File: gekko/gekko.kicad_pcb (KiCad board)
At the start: 2 copper layers, 58 x 60.5 mm, 89 parts, among them J1 Conn_01x02_Male, J2 Conn_01x04_Female, J3 Conn_01x05, J4 Conn_01x03, J5 Conn_01x02_Male, J6 Conn_01x02, J7 Conn_01x04_Female, J8 Conn_01x02_Male, J9 Conn_01x02_Male, Q5 IRLML6344TRPBFTR, SW1 SW_Push_Dual_x2, SW2 SW_DPDT_x2, U1 DRV8835, U10 MA702GQ-P, U11 MA702GQ-P, U12 sw_pch, U2 STM32F413CH6, U3 LED_FOTR, U4 LP5907_DBV, U5 ICM20648, U6 LED_FOTR, U7 LED_FOTR, U8 LED_FOTR, U9 RP124N334E-TR-FE, Y1 Crystal_GND23

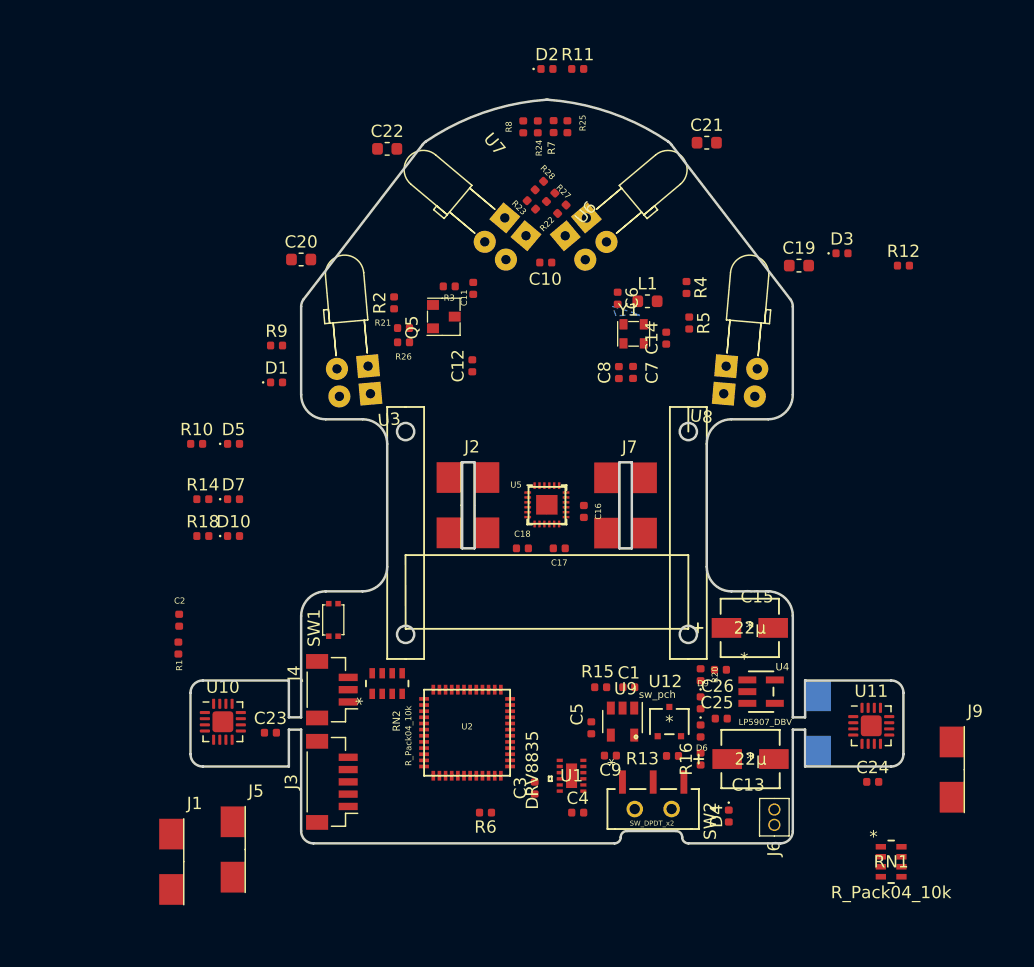
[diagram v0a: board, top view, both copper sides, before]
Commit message: betaGND
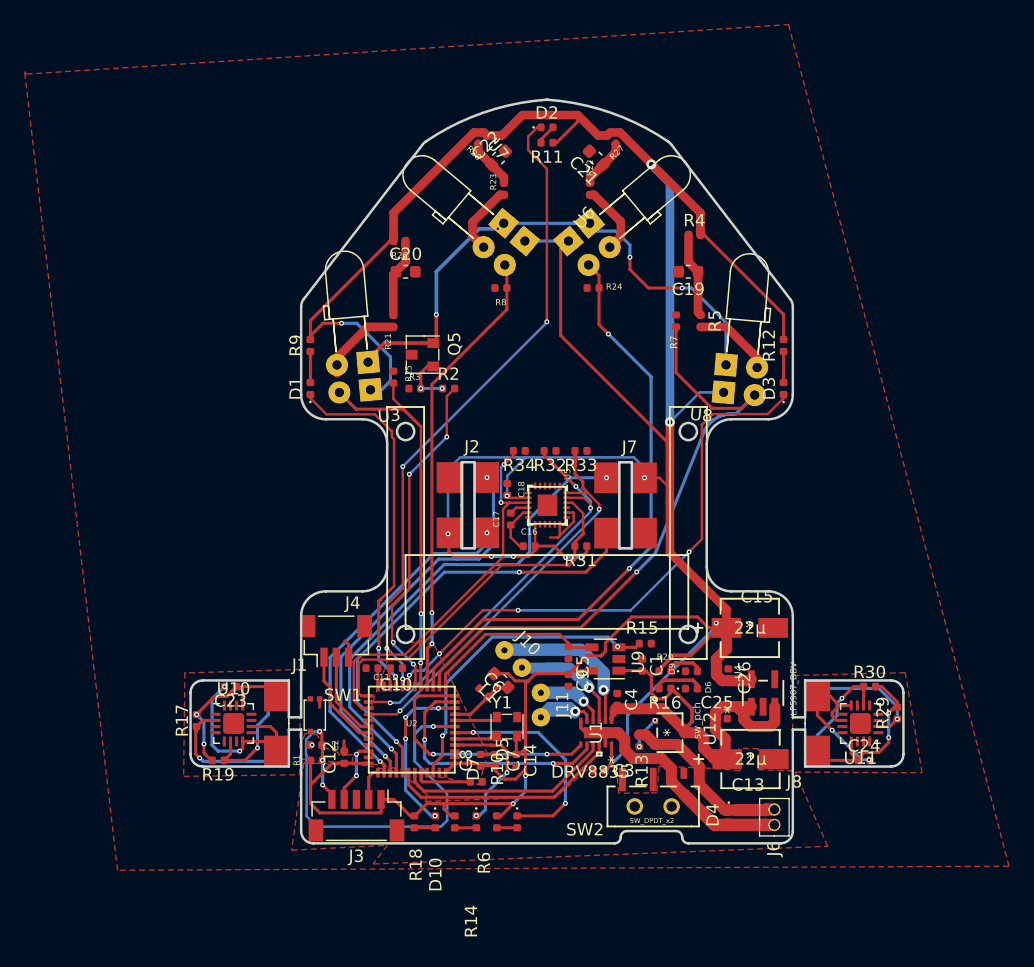
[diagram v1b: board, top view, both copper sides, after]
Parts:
- removed RN1, RN2: R_Pack04_10k, micro:R10k×4
- added J10: Conn_01x02, micro:motor_pad, F.Cu at (147.2, 132.3)
- added J11: Conn_01x02, micro:motor_pad, F.Cu at (149.5, 136.0)
- added R17: 10k, Resistor_SMD:R_0402_1005Metric, F.Cu at (121.5, 137.3)
- added R19: 10k, Resistor_SMD:R_0402_1005Metric, F.Cu at (123.2, 140.5)
- added R29: 10k, Resistor_SMD:R_0402_1005Metric, F.Cu at (178.5, 136.7)
- added R30: 10k, Resistor_SMD:R_0402_1005Metric, F.Cu at (176.2, 134.5)
- added R31: 10k, Resistor_SMD:R_0402_1005Metric, F.Cu at (152.7, 123.1)
- added R32: 10k, Resistor_SMD:R_0402_1005Metric, F.Cu at (150.2, 115.3)
- added R33: 10k, Resistor_SMD:R_0402_1005Metric, F.Cu at (152.8, 115.3)
- added R34: 10k, Resistor_SMD:R_0402_1005Metric, F.Cu at (147.7, 115.3)
- J5, J9: moved to B.Cu
- J8: moved to F.Cu
- moved R10 39.3 mm to (145.9, 145.5), turned to 270 degrees
- moved D5 38.4 mm to (147.6, 145.5), turned to 270 degrees
- moved C14 36.5 mm to (147.5, 140.5), turned to 270 degrees
- moved C10 35.2 mm to (137.7, 133.0)
- moved C6 33.9 mm to (144.8, 135.0), turned to 315 degrees
- moved Y1 33.6 mm to (146.7, 137.8)
- moved C12 33.5 mm to (133.5, 140.3)
- moved C7 33.5 mm to (145.7, 140.5)
- moved C8 33.5 mm to (144.6, 140.5)
- moved R14 33.3 mm to (142.5, 145.5), turned to 90 degrees
- moved L1 33.1 mm to (146.2, 134.0), turned to 135 degrees
- moved D7 32.9 mm to (144.2, 145.5), turned to 270 degrees
- moved C11 32.0 mm to (135.8, 133.0), turned to 180 degrees
- moved R18 28.9 mm to (139.2, 145.5), turned to 90 degrees
- moved D10 28.5 mm to (140.9, 145.5), turned to 270 degrees
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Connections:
- C23 pad 1: +3.3V -> +3.3V_L
- C23 pad 2: GND -> GND_L
- C24 pad 1: +3.3V -> +3.3V_R
- C24 pad 2: GND -> GND_R
- J1 pad 1: +3.3V -> +3.3V_L
- J1 pad 2: GND -> GND_L
- J2 pad 1: battery_wt_vout -> GND
- J2 pad 2: GND -> battery_wt_vout
- J7 pad 1: battery_wt_vout -> encR_2_EXTI
- J7 pad 2: GND -> encR_1_EXTI
- J7 pad 3: encR_1_EXTI -> battery_wt_vout
- J7 pad 4: encR_2_EXTI -> GND
- J8 pad 1: +3.3V -> +3.3V_R
- J8 pad 2: GND -> GND_R
- SW2 pad 1: Net-(SW2-Pad1) -> GND
- SW2 pad 3: GND -> Net-(SW2-Pad3)
- U1 pad 2: MotorR_Foward -> MotorR_Foward_Out
- U1 pad 3: MotorR_Reverce -> MotorR_Reverce_Out
- U1 pad 4: MotorL_Foward -> MotorL_Foward_Out
- U1 pad 5: MotorL_Reverce -> MotorL_Reverce_Out
- U10 pad 10: GND -> GND_L
- U10 pad 13: +3.3V -> +3.3V_L
- U10 pad 8: GND -> GND_L
- U11 pad 10: GND -> GND_R
- U11 pad 13: +3.3V -> +3.3V_R
- U11 pad 8: GND -> GND_R
- U2 pad 19: DEBUG_LED4 -> DEBUG_LED6
- U2 pad 21: DEBUG_LED6 -> DEBUG_LED4
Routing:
- net battery_wt_vout: track 0.00 -> 302.4 mm, vias 0 -> 14
- net DEBUG_LED5: track 0.00 -> 52.7 mm, vias 0 -> 4
- net sens_RR: track 0.00 -> 50.8 mm, vias 0 -> 1
- net sens_R: track 0.00 -> 48.3 mm, vias 0 -> 2
- net DEBUG_LED6: track 0.00 -> 46.8 mm, vias 0 -> 4
- net Net-(Q5-Pad2): track 0.00 -> 45.8 mm, vias 0 -> 4
- net encR_2_EXTI: track 0.00 -> 39.8 mm, vias 0 -> 2
- net BATT_SW: track 0.00 -> 39.2 mm
- net GND: track 0.00 -> 39.1 mm, vias 0 -> 1
- net NRST: track 0.00 -> 37.2 mm, vias 0 -> 4
- net sens_L: track 0.00 -> 37.1 mm, vias 0 -> 2
- net encR_1_EXTI: track 0.00 -> 36.1 mm, vias 0 -> 2
- net MOSI_IMU: track 0.00 -> 34.4 mm, vias 0 -> 2
- net SCK_IMU: track 0.00 -> 33.5 mm, vias 0 -> 3
- net encL_1_EXTI: track 0.00 -> 32.9 mm, vias 0 -> 2
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- added copper zone on F.Cu, net (none)
- removed copper zone on B.Cu, net GND
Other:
- rule via_min_drill: 0.3 -> 0.1
- rule via_min_size: 0.4 -> 0.2
